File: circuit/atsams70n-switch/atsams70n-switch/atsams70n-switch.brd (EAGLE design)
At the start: 176.5 x 171.7 mm, 72 parts, among them J5 CONN_20X2, Q1 20MHz, U1 REGULATOR_SOT223, U2 ATSAMS70N-TQFP100, U3 ISL3177E, U4 ISL3177E, U5 ISL3177E, U6 ISL3177E, X1 MICRO-USB_1/100

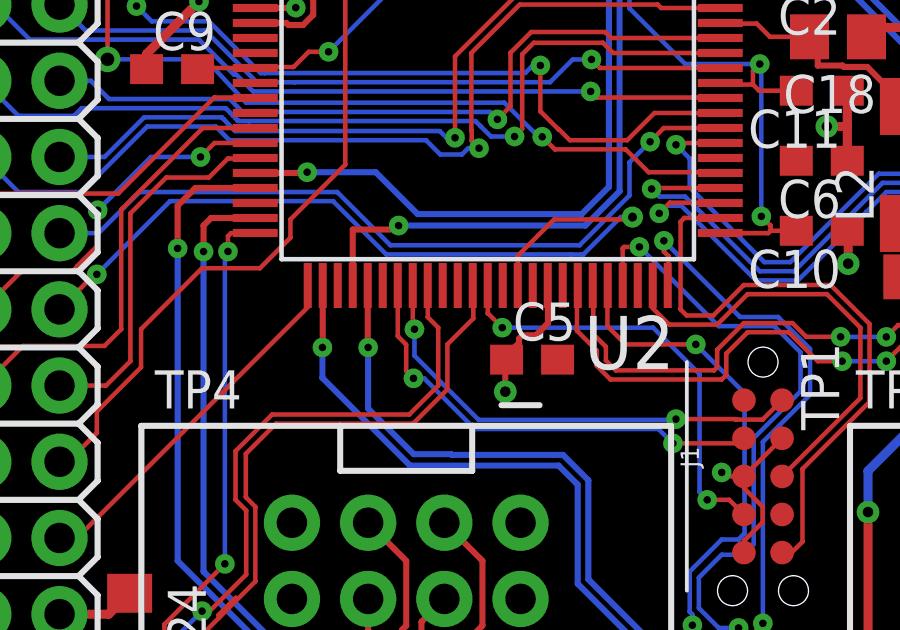
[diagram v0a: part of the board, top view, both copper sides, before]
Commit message: remove cdc
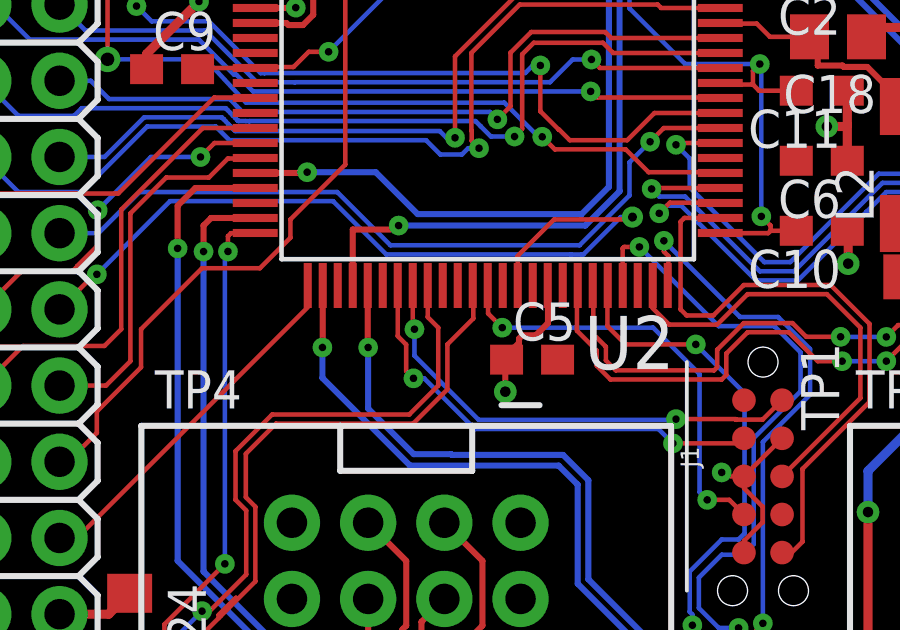
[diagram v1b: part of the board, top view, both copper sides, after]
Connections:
- net TCK renamed TCK/SWCLK
- net TMS renamed TMS/SWDIO
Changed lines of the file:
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@@
 <wire x1="47.522253125" y1="37.3937625" x2="48.475" y2="37.2413625" width="0.2032" layer="1"/>
-</signal>
-<signal name="TCK">
-<contactref element="U2" pad="63"/>
-<contactref element="TP1" pad="4"/>
-<wire x1="42.24568125" y1="23.64269375" x2="41.758375" y2="24.13" width="0.1524" layer="1"/>
-<wire x1="41.758375" y1="24.13" x2="41.021" y2="24.13" width="0.1524" layer="1"/>
-<wire x1="33.704959375" y1="31.2762" x2="33.704959375" y2="30.343209375" width="0.1524" layer="1"/>
-<wire x1="33.704959375" y1="30.343209375" x2="33.715590625" y2="30.343209375" width="0.1524" layer="1"/>
-<wire x1="33.715590625" y1="30.343209375" x2="34.1884" y2="29.8704" width="0.1524" layer="1"/>
-<via x="34.1884" y="29.8704" extent="1-16" drill="0.25"/>
-<wire x1="39.2176" y1="29.8704" x2="40.767" y2="28.321" width="0.1524" layer="16"/>
-<wire x1="34.1884" y1="29.8704" x2="39.2176" y2="29.8704" width="0.1524" layer="16"/>
-<via x="41.021" y="24.13" extent="1-16" drill="0.25"/>
-<wire x1="40.767" y1="28.321" x2="40.767" y2="24.384" width="0.1524" layer="16"/>
-<wire x1="40.767" y1="24.384" x2="41.021" y2="24.13" width="0.1524" layer="16"/>
-</signal>
-<signal name="TMS">
-<contactref element="U2" pad="57"/>
-<contactref element="TP1" pad="2"/>
-<wire x1="30.704959375" y1="31.2762" x2="30.704959375" y2="29.588971875" width="0.1524" layer="1"/>
-<wire x1="30.704959375" y1="29.588971875" x2="30.985165625" y2="29.308765625" width="0.1524" layer="1"/>
-<wire x1="30.985165625" y1="29.308765625" x2="30.985165625" y2="28.425396875" width="0.1524" layer="1"/>
-<wire x1="30.985165625" y1="28.425396875" x2="31.22928125" y2="28.18128125" width="0.1524" layer="1"/>
-<via x="31.22928125" y="28.18128125" extent="1-16" drill="0.25"/>
-<wire x1="31.22928125" y1="28.18128125" x2="31.5856625" y2="28.18128125" width="0.1524" layer="16"/>
-<wire x1="39.3954" y1="26.4922" x2="39.7256" y2="26.162" width="0.1524" layer="16"/>
-<wire x1="33.27474375" y1="26.4922" x2="39.3954" y2="26.4922" width="0.1524" layer="16"/>
-<wire x1="39.7256" y1="26.162" x2="39.7296" y2="26.162" width="0.1524" layer="16"/>
-<wire x1="39.7296" y1="26.162" x2="39.878" y2="26.0136" width="0.1524" layer="16"/>
-<via x="39.878" y="26.0136" extent="1-16" drill="0.25"/>
-<wire x1="39.878" y1="26.0136" x2="42.0765875" y2="26.0136" width="0.1524" layer="1"/>
-<wire x1="42.0765875" y1="26.0136" x2="42.24568125" y2="26.18269375" width="0.1524" layer="1"/>
-<wire x1="31.5856625" y1="28.18128125" x2="33.27474375" y2="26.4922" width="0.1524" layer="16"/>
 </signal>
 <signal name="TDO">
@@
 <wire x1="14.478" y1="52.4764" x2="14.478" y2="59.0804" width="0" layer="19" extent="1-1"/>
 </signal>
+<signal name="TCK/SWCLK">
+<contactref element="U2" pad="63"/>
+<contactref element="TP1" pad="4"/>
+<wire x1="42.24568125" y1="23.64269375" x2="41.758375" y2="24.13" width="0.1524" layer="1"/>
+<wire x1="41.758375" y1="24.13" x2="41.021" y2="24.13" width="0.1524" layer="1"/>
+<wire x1="34.1884" y1="29.8704" x2="33.715590625" y2="30.343209375" width="0.1524" layer="1"/>
+<via x="34.1884" y="29.8704" extent="1-16" drill="0.25"/>
+<wire x1="39.2176" y1="29.8704" x2="40.767" y2="28.321" width="0.1524" layer="16"/>
+<wire x1="34.1884" y1="29.8704" x2="39.2176" y2="29.8704" width="0.1524" layer="16"/>
+<via x="41.021" y="24.13" extent="1-16" drill="0.25"/>
+<wire x1="40.767" y1="28.321" x2="40.767" y2="24.384" width="0.1524" layer="16"/>
+<wire x1="40.767" y1="24.384" x2="41.021" y2="24.13" width="0.1524" layer="16"/>
+<wire x1="33.715590625" y1="31.26556875" x2="33.704959375" y2="31.2762" width="0.1524" layer="1"/>
+<wire x1="33.715590625" y1="30.343209375" x2="33.715590625" y2="31.26556875" width="0.1524" layer="1"/>
+</signal>
+<signal name="TMS/SWDIO">
+<contactref element="U2" pad="57"/>
+<contactref element="TP1" pad="2"/>
+<wire x1="30.985165625" y1="29.308765625" x2="30.704959375" y2="29.588971875" width="0.1524" layer="1"/>
+<wire x1="30.985165625" y1="29.308765625" x2="30.985165625" y2="28.425396875" width="0.1524" layer="1"/>
+<wire x1="30.985165625" y1="28.425396875" x2="31.22928125" y2="28.18128125" width="0.1524" layer="1"/>
+<via x="31.22928125" y="28.18128125" extent="1-16" drill="0.25"/>
+<wire x1="31.22928125" y1="28.18128125" x2="31.5856625" y2="28.18128125" width="0.1524" layer="16"/>
+<wire x1="39.3954" y1="26.4922" x2="39.7256" y2="26.162" width="0.1524" layer="16"/>
+<wire x1="33.27474375" y1="26.4922" x2="39.3954" y2="26.4922" width="0.1524" layer="16"/>
+<wire x1="39.7256" y1="26.162" x2="39.7296" y2="26.162" width="0.1524" layer="16"/>
+<wire x1="39.7296" y1="26.162" x2="39.878" y2="26.0136" width="0.1524" layer="16"/>
+<via x="39.878" y="26.0136" extent="1-16" drill="0.25"/>
+<wire x1="39.878" y1="26.0136" x2="42.0765875" y2="26.0136" width="0.1524" layer="1"/>
+<wire x1="42.0765875" y1="26.0136" x2="42.24568125" y2="26.18269375" width="0.1524" layer="1"/>
+<wire x1="31.5856625" y1="28.18128125" x2="33.27474375" y2="26.4922" width="0.1524" layer="16"/>
+<wire x1="30.704959375" y1="29.588971875" x2="30.704959375" y2="31.2762" width="0.1524" layer="1"/>
+</signal>
 </signals>
